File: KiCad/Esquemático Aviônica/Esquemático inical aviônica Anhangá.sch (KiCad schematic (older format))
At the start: 21 parts, among them J1 Conn_01x06_Female, J2 Conn_01x06_Female, J3 Conn_01x12_Female, J4 Conn_01x12_Female, J5 Screw_Terminal_01x02, J6 Conn_01x06_Male, J7 Screw_Terminal_01x02, J8 Conn_01x07_Female, J9 Conn_01x06_Male, Q1 IRF7403, U1 ME620933

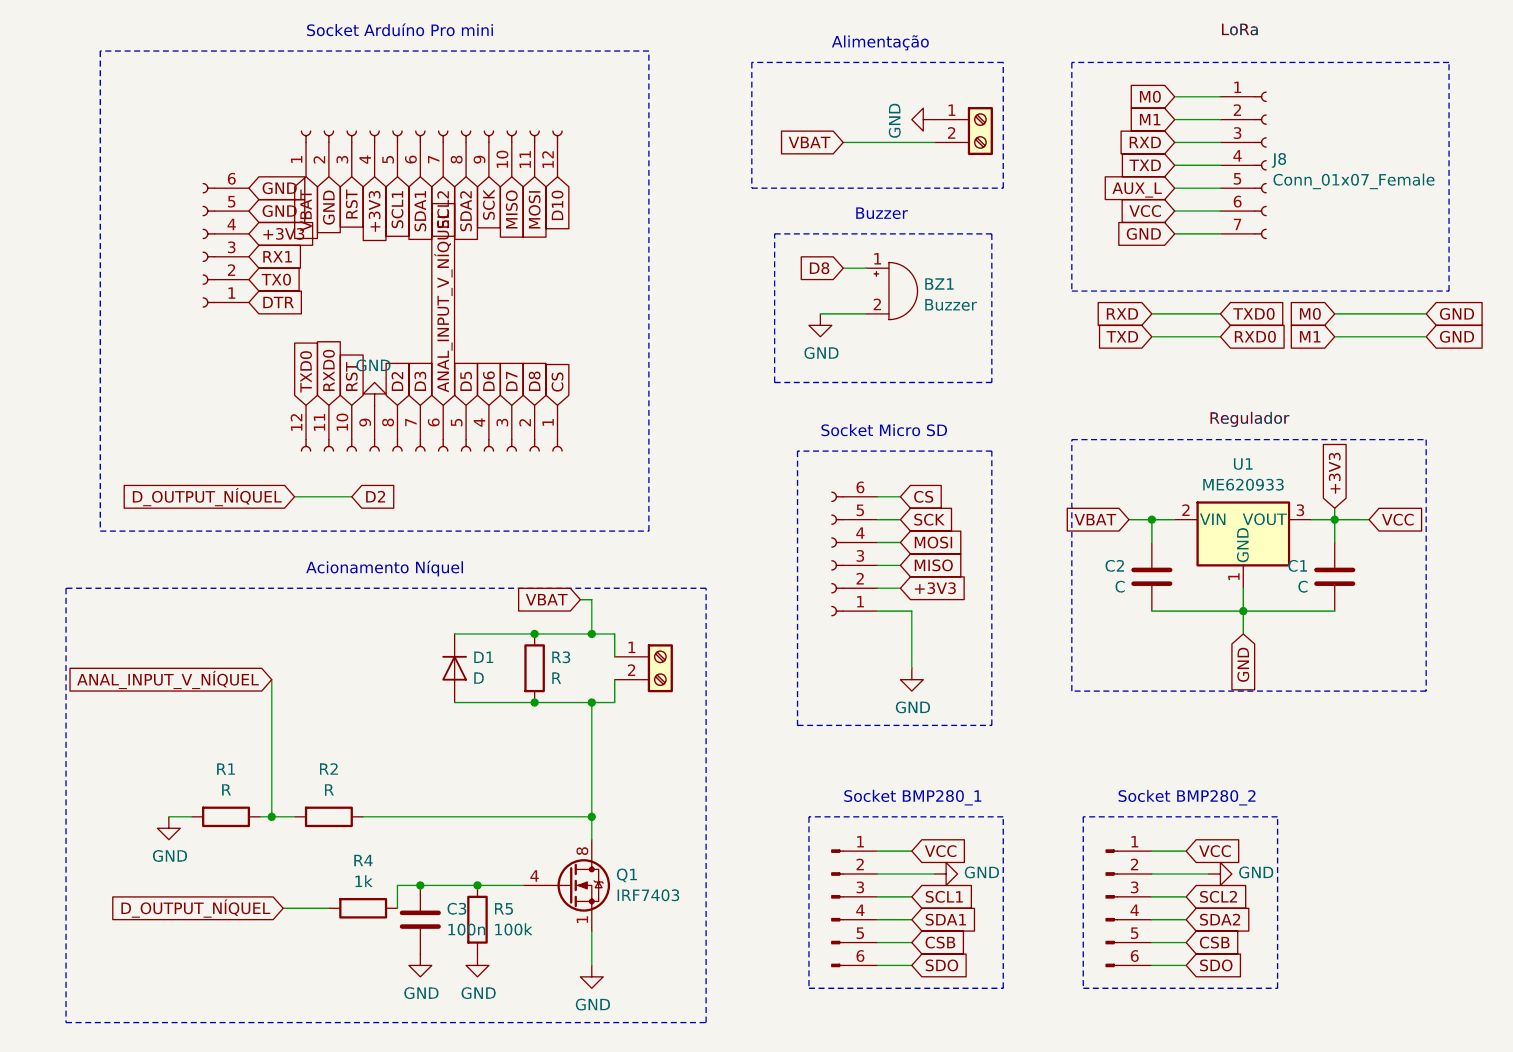
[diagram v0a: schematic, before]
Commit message: Atualização Layout
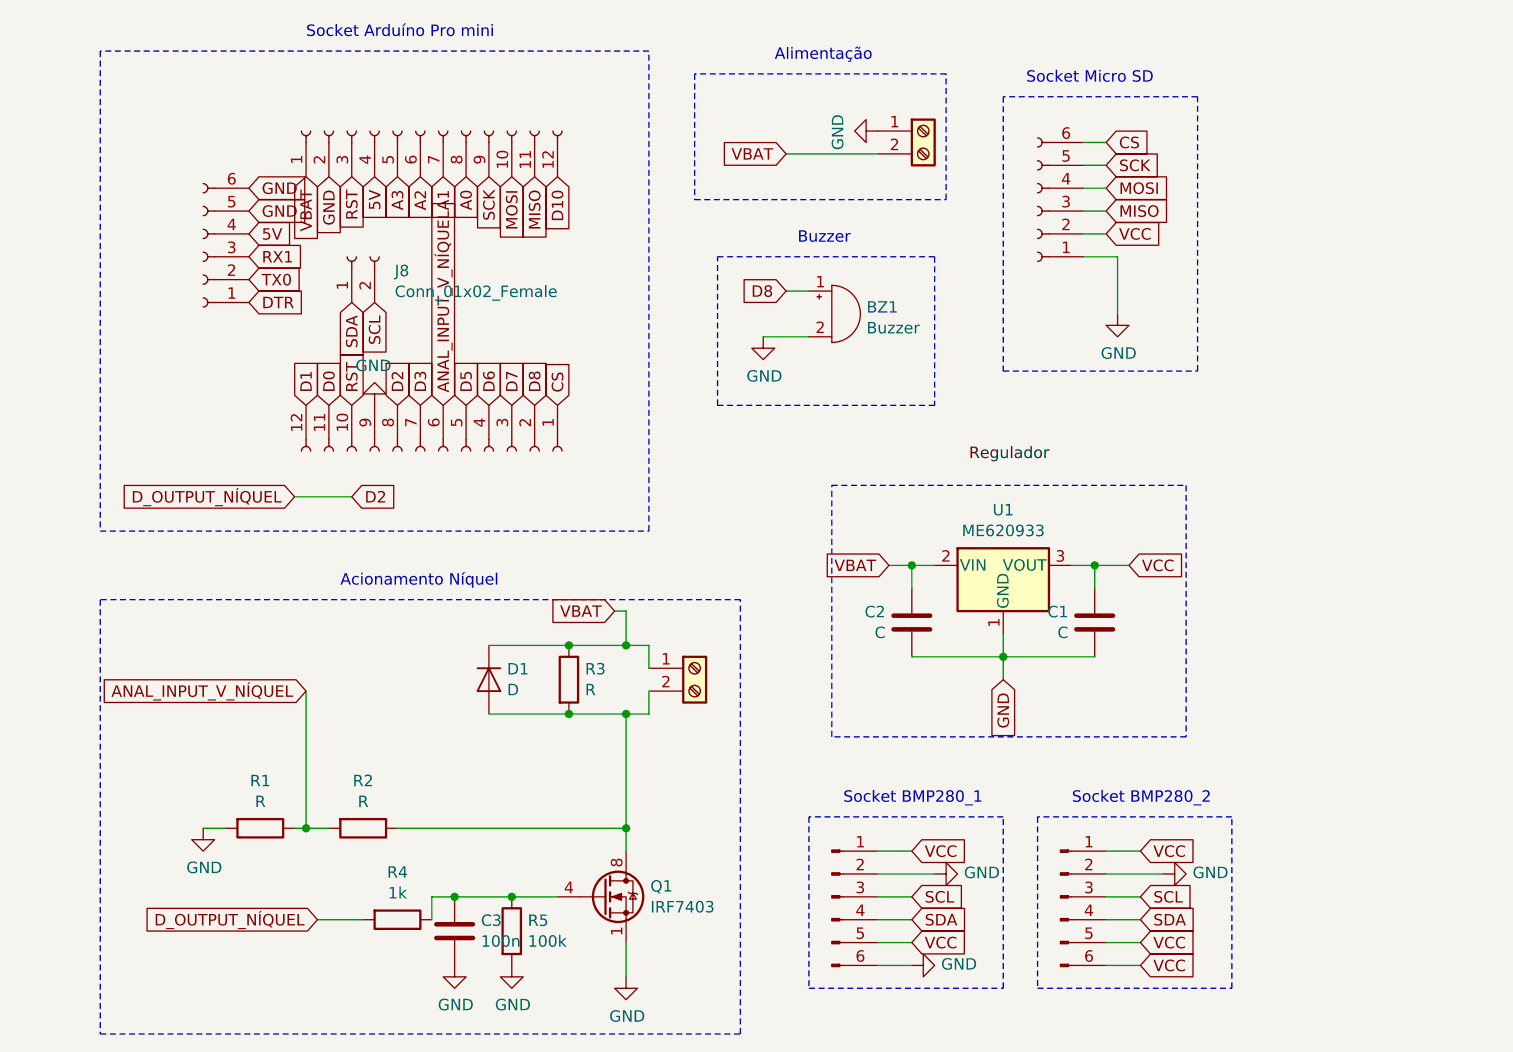
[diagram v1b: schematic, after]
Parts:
- removed J8: Conn_01x07_Female, Connector_PinSocket_2.54mm:PinSocket_1x07_P2.54mm_Vertical, symbol Connector:Conn_01x07_Female
- added J8: Conn_01x02_Female, Connector_PinSocket_2.54mm:PinSocket_1x02_P2.54mm_Vertical, symbol Connector:Conn_01x02_Female
- R1, R2, R3, R4, R5: footprint Resistor_SMD:R_0805_2012Metric_Pad1.15x1.40mm_HandSolder -> Resistor_THT:R_Axial_DIN0207_L6.3mm_D2.5mm_P5.08mm_Vertical
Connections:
- net CSB is gone; now on net VCC: J6.5 (Pin_5), J9.5 (Pin_5)
- net GND: now also J9.6 (Pin_6)
- net MISO: now also J3.11 (Pin_11); no longer J3.10 (Pin_10)
- net MOSI: now also J3.10 (Pin_10); no longer J3.11 (Pin_11)
- net +3V3 renamed VCC
- net VCC: now also J6.6 (Pin_6); no longer J2.4 (Pin_4), J3.4 (Pin_4)
- net RXD renamed D1
- net RXD0 renamed D0
- net SCL1 renamed A3
- net A3: no longer J9.3 (Pin_3)
- net SCL2 renamed A1
- net A1: no longer J6.3 (Pin_3)
- net SDA1 renamed A2
- net A2: no longer J9.4 (Pin_4)
- net SDA2 renamed A0
- net A0: no longer J6.4 (Pin_4)
- removed net SDO: J6.6 (Pin_6), J9.6 (Pin_6)
- new net 5V: J2.4 (Pin_4), J3.4 (Pin_4)
- new net SCL: J6.3 (Pin_3), J8.2 (Pin_2), J9.3 (Pin_3)
- new net SDA: J6.4 (Pin_4), J8.1 (Pin_1), J9.4 (Pin_4)
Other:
- moved on the sheet: BZ1, C1, C2, C3, D1, Q1, R1, R2, R3, R4, R5, U1

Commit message: Atualização Layout
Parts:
- J6, J9: footprint Connector_PinHeader_2.54mm:PinHeader_1x06_P2.54mm_Vertical -> Connector_PinSocket_2.54mm:PinSocket_1x06_P2.54mm_Vertical
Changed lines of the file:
@@
 F 0 "J6" H 5758 6389 50  0001 C CNN
 F 1 "Conn_01x06_Male" H 5758 6390 50  0001 C CNN
-F 2 "Connector_PinHeader_2.54mm:PinHeader_1x06_P2.54mm_Vertical" H 5650 6100 50  0001 C CNN
+F 2 "Connector_PinSocket_2.54mm:PinSocket_1x06_P2.54mm_Vertical" H 5650 6100 50  0001 C CNN
 F 3 "~" H 5650 6100 50  0001 C CNN
 	1    5650 6100
@@
 F 0 "J9" H 4758 6389 50  0001 C CNN
 F 1 "Conn_01x06_Male" H 4758 6390 50  0001 C CNN
-F 2 "Connector_PinHeader_2.54mm:PinHeader_1x06_P2.54mm_Vertical" H 4650 6100 50  0001 C CNN
+F 2 "Connector_PinSocket_2.54mm:PinSocket_1x06_P2.54mm_Vertical" H 4650 6100 50  0001 C CNN
 F 3 "~" H 4650 6100 50  0001 C CNN
 	1    4650 6100

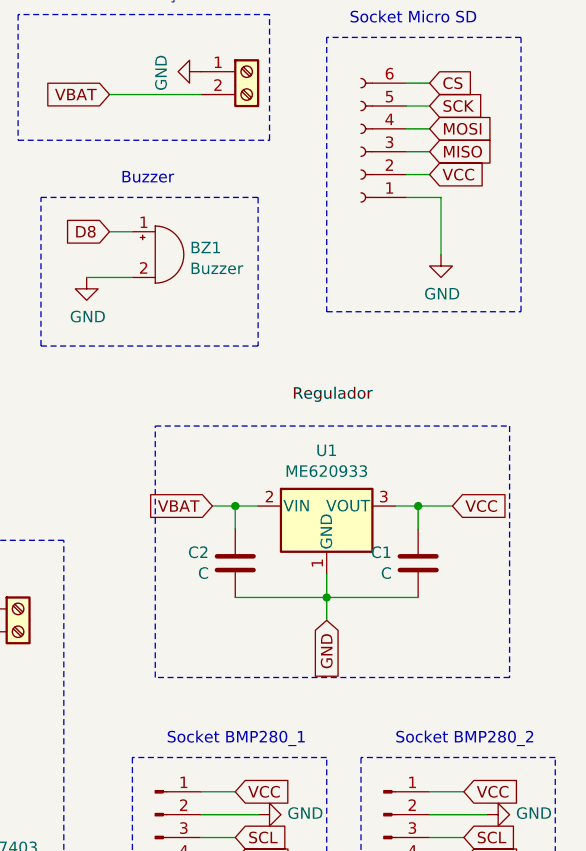
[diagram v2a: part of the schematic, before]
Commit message: Atual. Layout + Esquemát.
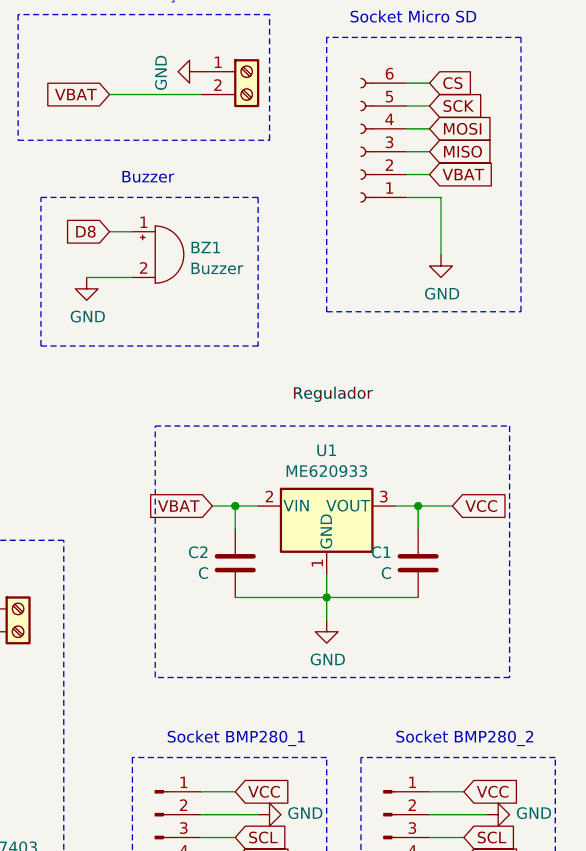
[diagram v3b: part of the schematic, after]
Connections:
- net VBAT: now also J1.2 (Pin_2)
- net VCC: no longer J1.2 (Pin_2)
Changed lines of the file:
@@
 VBAT
 Text GLabel 5850 3200 2    50   Input ~ 0
-VCC
+VBAT
 Wire Notes Line
 	1450 2400 1450 4500
@@
 Wire Notes Line
 	6200 5400 4650 5400
-Text GLabel 5400 5150 3    50   Input ~ 0
-GND
 Text GLabel 4900 4650 0    50   Input ~ 0
 VBAT
@@
 Text GLabel 3250 2950 3    50   Input ~ 0
 MOSI
+$Comp
+L power:GND #PWR?
+U 1 1 5DB38D1B
+P 5400 5150
+F 0 "#PWR?" H 5400 4900 50  0001 C CNN
+F 1 "GND" H 5405 4977 50  0000 C CNN
+F 2 "" H 5400 5150 50  0001 C CNN
+F 3 "" H 5400 5150 50  0001 C CNN
+	1    5400 5150
+	1    0    0    -1
+$EndComp
 $EndSCHEMATC
